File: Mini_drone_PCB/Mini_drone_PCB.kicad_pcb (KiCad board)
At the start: 2 copper layers, 45.7 x 42.9 mm, 56 parts, among them J1 XT30PW-M, Q1 SS8050, Q2 SS8050, Q3 AO3400, Q4 AO3400, Q5 AO3400, Q6 AO3400, Q7 AO4407A, SW1 SW_Push, SW2 Slide_switch, U1 TPS62085RLTR, U2 470nH 6.9mΩ, U3 ESP32-S3-MINI-1, U4 MPU-6050, U5 CH343P, U6 INA236AIDDFR, U7 USBLC6-2P6

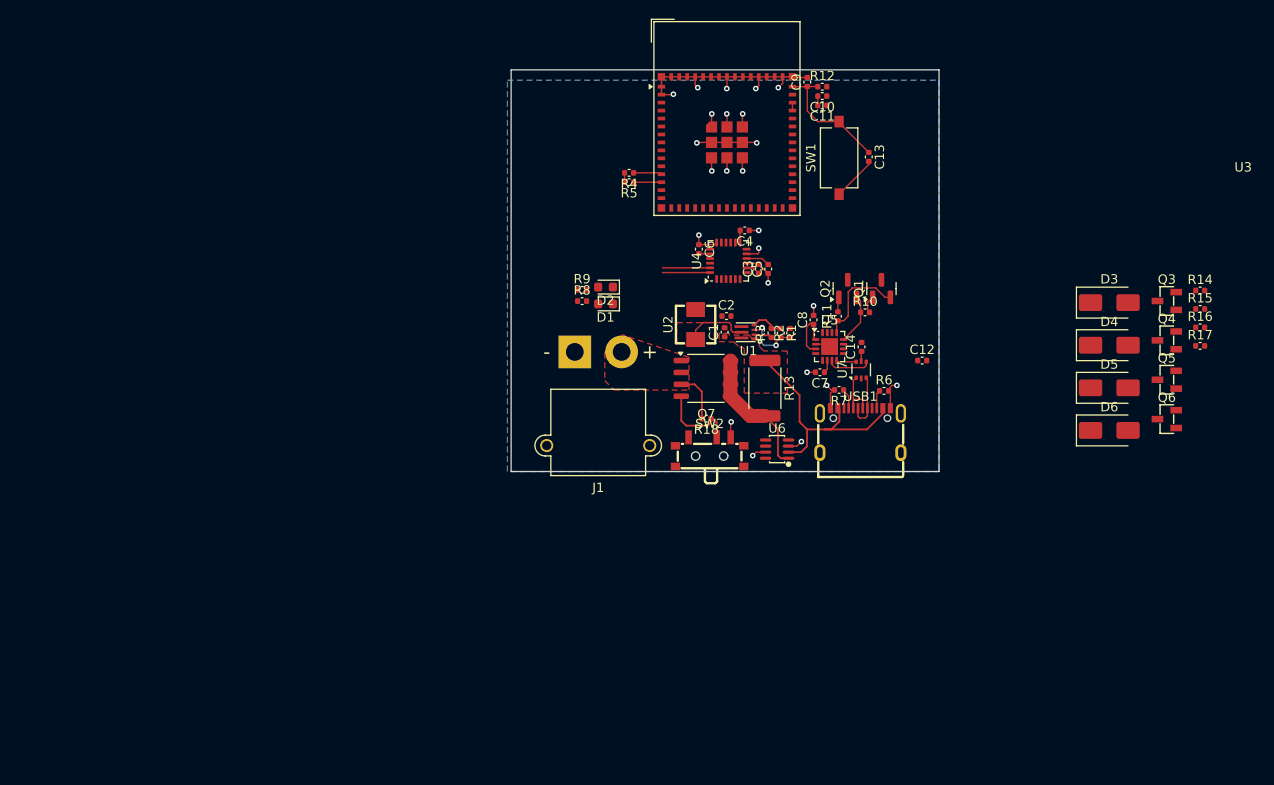
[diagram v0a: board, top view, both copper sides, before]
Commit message: update_sch_and_PCB
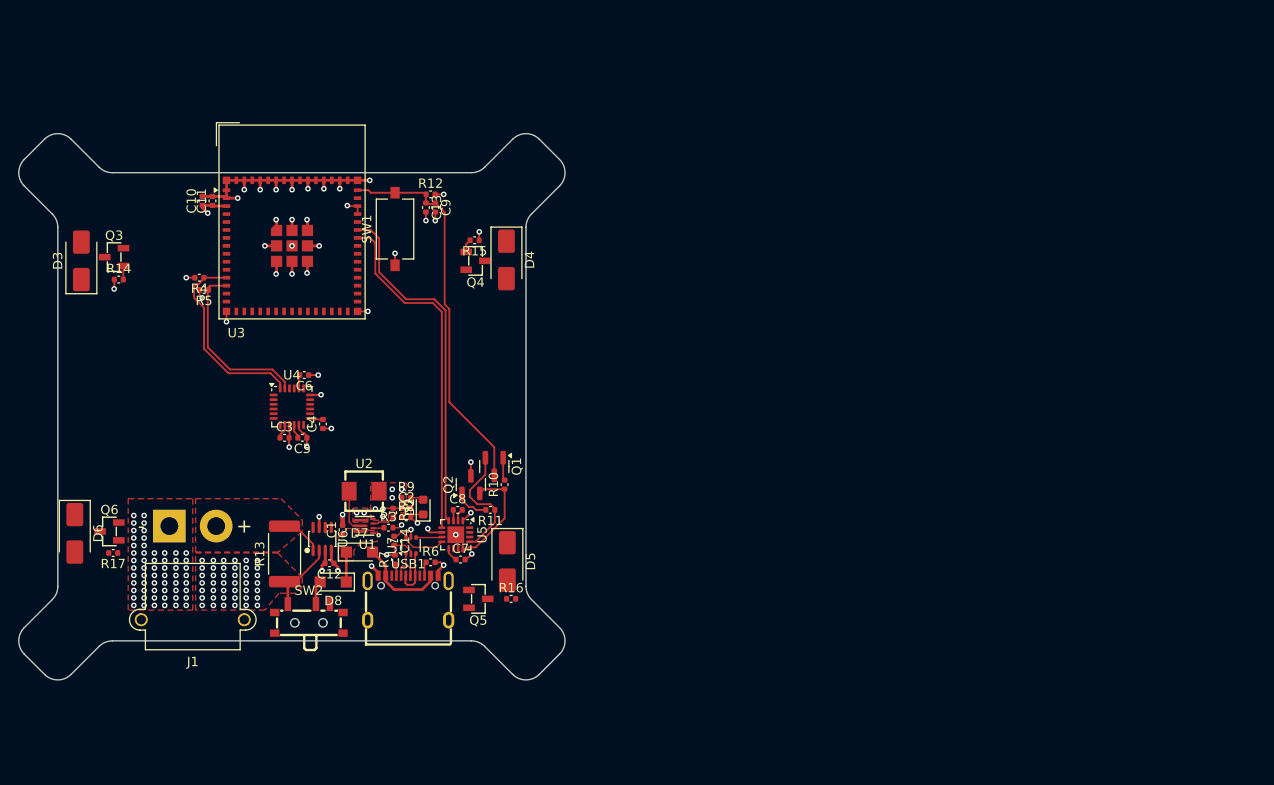
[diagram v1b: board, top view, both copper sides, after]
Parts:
- removed D1: VBAT LED, LED_SMD:LED_0603_1608Metric
- removed Q7: AO4407A, mini_drone:AO4407A
- removed R18: 10k, Capacitor_SMD:C_0402_1005Metric
- removed R8: 510, Capacitor_SMD:C_0402_1005Metric
- added D7: PMEG2010ER, Diode_SMD:Nexperia_CFP3_SOD-123W, F.Cu at (106.8, 115.1)
- added D8: PMEG2010ER, Diode_SMD:Nexperia_CFP3_SOD-123W, F.Cu at (104.0, 118.3)
- moved R17 118.2 mm to (80.5, 115.2), turned to 180 degrees
- moved R14 115.5 mm to (81.1, 86.0)
- moved Q6 113.6 mm to (80.1, 112.9)
- moved Q3 112.5 mm to (80.6, 83.6)
- moved D6 111.0 mm to (76.4, 113.1), turned to -90 degrees
- moved D3 109.9 mm to (77.1, 84.0), turned to 90 degrees
- moved R16 79.1 mm to (123.0, 120.1)
- moved R15 77.8 mm to (119.1, 81.8), turned to 180 degrees
- moved Q5 77.2 mm to (119.5, 120.1), turned to 180 degrees
- moved Q4 74.3 mm to (119.2, 84.0), turned to 180 degrees
- moved C10 67.1 mm to (90.0, 77.6), turned to 90 degrees
- moved D5 66.9 mm to (122.6, 116.1), turned to -90 degrees
- moved C12 66.9 mm to (103.6, 116.3), turned to 180 degrees
- moved C11 65.9 mm to (91.1, 77.6), turned to 90 degrees
- moved D4 65.0 mm to (122.5, 83.9), turned to -90 degrees
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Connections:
- C1 pad 1: +BATT -> +VIN
- C14 pad 1: +BATT -> +VBUS
- R13 pad 2: Net-(Q7-D) -> Net-(J1-+)
- SW2 pad 1: unconnected-(SW2-Pad1) -> +BATT
- SW2 pad 3: GND -> unconnected-(SW2-Pad3)
- U1 pad 1: +BATT -> +VIN
- U1 pad 7: +BATT -> +VIN
- U6 pad 1: Net-(Q7-D) -> Net-(J1-+)
- U7 pad 5: +BATT -> +VBUS
- USB1 pad 11: +BATT -> +VBUS
- USB1 pad 2: +BATT -> +VBUS
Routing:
- net /MCU/U0RXD: track 0.00 -> 37.7 mm
- net /MCU/U0TXD: track 0.00 -> 37.2 mm
- net /MCU/CHIP_PU: track 13.8 -> 41.1 mm
- net +BATT: track 27.1 -> 7.59 mm, vias 0 -> 42
- net Net-(Q7-D): track 14.4 -> 0.00 mm
- net /MCU/ESP_SDA: track 8.13 -> 21.2 mm
- net +VBUS: track 0.00 -> 12.7 mm, vias 0 -> 1
- net /MCU/ESP_SCL: track 8.07 -> 18.9 mm
- net +3V3: track 14.6 -> 21.9 mm, vias 0 -> 14
- net Net-(D8-A): track 8.93 -> 2.55 mm
- net /MCU/DTR: track 5.51 -> 11.8 mm
- net GND: track 69.6 -> 74.1 mm, vias 24 -> 100
- net Net-(U1-FB): track 6.28 -> 2.43 mm, vias 2 -> 0
- net +VIN: track 0.00 -> 2.90 mm
- net /MCU/RTS: track 10.3 -> 13.1 mm
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- added copper zone on F.Cu, net +3V3
- added copper zone on F.Cu, net +VIN
- added copper zone on F.Cu, net GND
- removed copper zone on B.Cu, net GND
- removed copper zone on F.Cu, net Net-(U1-SW)
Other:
- board size 45.7 x 42.9 mm -> 58.3 x 58.3 mm

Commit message: Route_Finished
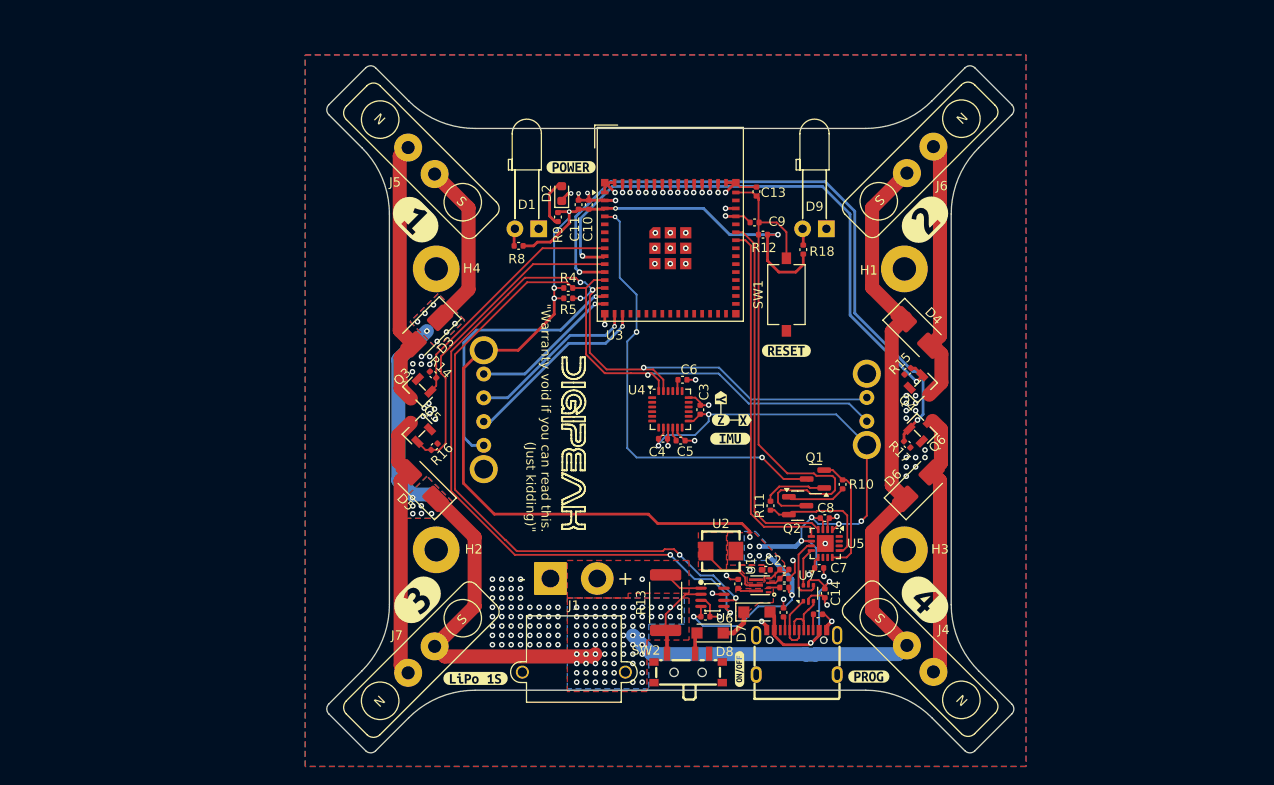
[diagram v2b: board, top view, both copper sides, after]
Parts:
- added D1: LED, LED_THT:LED_D3.0mm_Horizontal_O6.35mm_Z2.0mm, F.Cu at (125.9, 80.6)
- added D9: LED, LED_THT:LED_D3.0mm_Horizontal_O6.35mm_Z2.0mm, F.Cu at (156.7, 80.6)
- added H1: MountingHole_Pad, MountingHole:MountingHole_2.5mm_Pad, F.Cu at (165.0, 84.9)
- added H2: MountingHole_Pad, MountingHole:MountingHole_2.5mm_Pad, F.Cu at (115.0, 114.9)
- added H3: MountingHole_Pad, MountingHole:MountingHole_2.5mm_Pad, F.Cu at (165.0, 114.9)
- added H4: MountingHole_Pad, MountingHole:MountingHole_2.5mm_Pad, F.Cu at (115.0, 84.9)
- added J2: VL53L1X ToF Pogo, mini_drone:POGO 4Pin Pitch 2.54, B.Cu at (155.9, 101.1)
- added J3: PMW3901 Optical Flow Pogo, mini_drone:POGO 6Pin Pitch 2.54, B.Cu at (125.2, 96.1)
- added J4: Motor4_Pogo, mini_drone:POGO 2Pin Pitch 4, F.Cu at (169.9, 122.6)
- added J5: Motor1_Pogo, mini_drone:POGO 2Pin Pitch 4, F.Cu at (110.2, 77.2)
- added J6: Motor2_Pogo, mini_drone:POGO 2Pin Pitch 4, F.Cu at (162.8, 70.0)
- added J7: Motor3_Pogo, mini_drone:POGO 2Pin Pitch 4, F.Cu at (117.3, 129.8)
- added R18: 510, Capacitor_SMD:C_0402_1005Metric, F.Cu at (154.2, 82.8)
- added R8: 510, Capacitor_SMD:C_0402_1005Metric, F.Cu at (123.8, 82.4)
- added kibuzzard-696EF072: G***, kibuzzard-696EF072, F.Cu at (119.2, 128.6)
- added kibuzzard-696EF0B2: G***, kibuzzard-696EF0B2, F.Cu at (161.2, 128.4)
- added kibuzzard-696EF12B: G***, kibuzzard-696EF12B, F.Cu at (112.8, 79.6)
- added kibuzzard-696EF142: G***, kibuzzard-696EF142, F.Cu at (167.2, 79.6)
- added kibuzzard-696EF14F: G***, kibuzzard-696EF14F, F.Cu at (113.0, 120.2)
- added kibuzzard-696EF15F: G***, kibuzzard-696EF15F, F.Cu at (167.2, 120.2)
- added kibuzzard-696EF1CC: G***, kibuzzard-696EF1CC, F.Cu at (147.4, 127.6)
- added kibuzzard-696EF1EE: G***, kibuzzard-696EF1EE, F.Cu at (152.4, 93.6)
- added kibuzzard-696EF202: G***, kibuzzard-696EF202, F.Cu at (129.4, 74.0)
- added kibuzzard-696EF46D: G***, kibuzzard-696EF46D, B.Cu at (124.4, 100.0)
- added kibuzzard-696EF488: G***, kibuzzard-696EF488, B.Cu at (156.8, 100.0)
- added kibuzzard-696EFAC1: G***, kibuzzard-696EFAC1, F.Cu at (148.0, 101.0)
- added kibuzzard-696EFAE6: G***, kibuzzard-696EFAE6, F.Cu at (145.4, 98.6)
- added kibuzzard-696EFB18: G***, kibuzzard-696EFB18, F.Cu at (145.4, 101.0)
- added kibuzzard-696EFB3D: G***, kibuzzard-696EFB3D, F.Cu at (146.4, 103.0)
- R9: value 220 -> 510
- moved D6 90.2 mm to (166.5, 108.0), turned to 45 degrees
- moved Q6 87.5 mm to (166.9, 101.9), turned to -135 degrees
- moved R17 85.6 mm to (165.3, 103.6), turned to 135 degrees
- moved Q4 49.6 mm to (166.9, 97.6), turned to 135 degrees
- moved R15 48.3 mm to (165.3, 95.8), turned to 45 degrees
- moved C14 46.3 mm to (156.5, 119.5)
- moved D4 44.5 mm to (166.3, 91.7), turned to -45 degrees
- moved C3 44.5 mm to (143.2, 99.9), turned to 90 degrees
- moved D7 42.9 mm to (149.2, 121.5)
- moved R3 42.8 mm to (152.2, 118.9)
- moved U7 42.8 mm to (154.8, 119.5)
- moved U1 42.7 mm to (149.8, 118.7)
- moved C1 42.6 mm to (147.2, 118.5)
- moved SW1 42.4 mm to (152.4, 87.6)
- moved R1 42.2 mm to (152.2, 117.0), turned to 0 degrees
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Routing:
- net +3V3: track 21.9 -> 199.0 mm, vias 14 -> 20
- net +BATT: track 7.59 -> 173.6 mm, vias 42 -> 89
- net /MCU/ESP_SCL: track 18.9 -> 117.5 mm, vias 0 -> 6
- net /MCU/ESP_SDA: track 21.2 -> 113.3 mm, vias 0 -> 3
- net /MCU/Motor4_PWM: track 0.00 -> 70.0 mm, vias 0 -> 2
- net /MCU/Motor2_PWM: track 1.42 -> 61.3 mm, vias 0 -> 2
- net /MCU/GPIO0: track 1.46 -> 48.0 mm, vias 1 -> 3
- net /MCU/Motor3_PWM: track 0.00 -> 34.8 mm
- net /MCU/ESP_CS: track 0.00 -> 29.7 mm, vias 0 -> 1
- net Net-(D3-A): track 0.00 -> 28.8 mm
- net Net-(D5-A): track 0.00 -> 28.4 mm
- net Net-(D6-A): track 0.00 -> 28.2 mm
- net Net-(D4-A): track 0.00 -> 28.1 mm
- net /MCU/Motor1_PWM: track 1.46 -> 26.9 mm
- net /MCU/ESP_MISO: track 0.00 -> 20.4 mm, vias 0 -> 1
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- added copper zone on B.Cu, net +3V3
- added copper zone on B.Cu, net +BATT
- added copper zone on B.Cu, net GND
- added copper zone on F.Cu, net Net-(U1-SW)
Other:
- board size 58.3 x 58.3 mm -> 73.4 x 73.4 mm
- board text added: "Offset"
- board text added: "{dblquote}Warranty void if you can read this. (Just kidding){dblquote}"

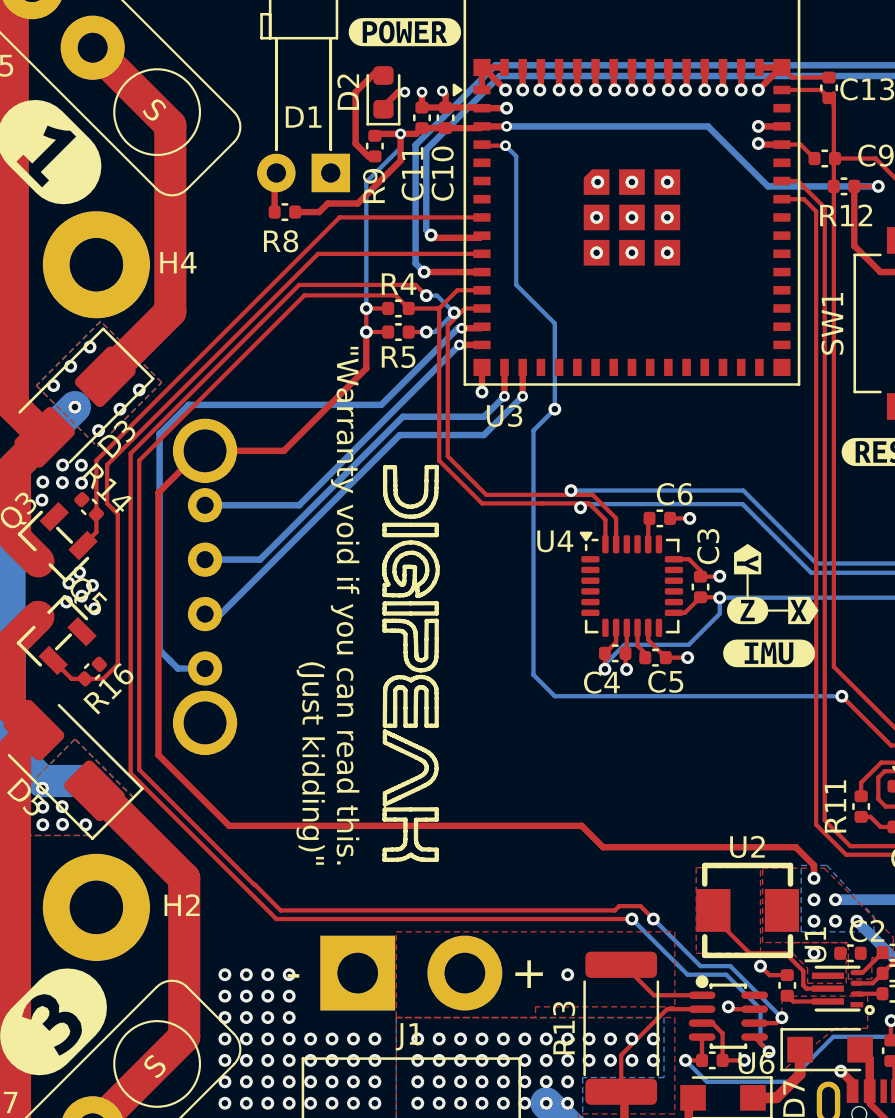
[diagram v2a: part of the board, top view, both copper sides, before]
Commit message: Verified and Finished
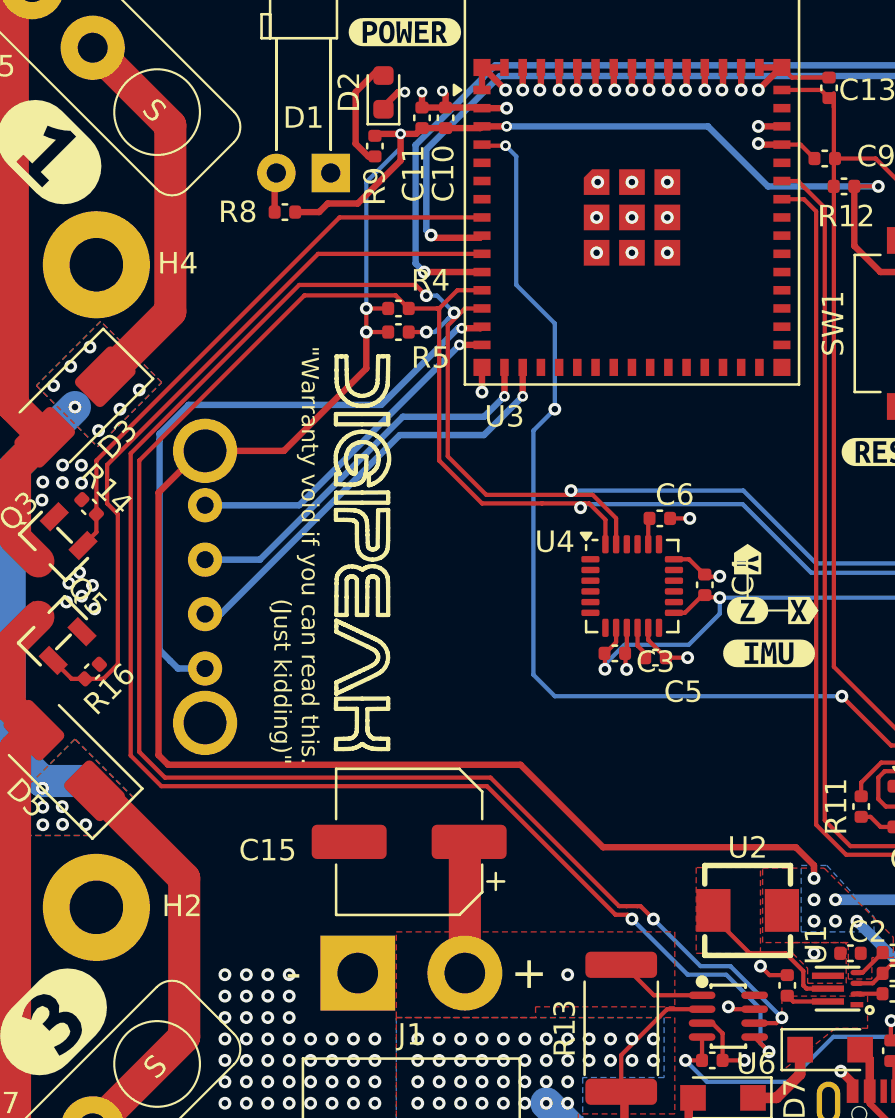
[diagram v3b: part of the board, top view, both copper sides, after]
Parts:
- added C15: 220uF, Capacitor_SMD:CP_Elec_6.3x5.4, F.Cu at (129.6, 111.8)
- moved C4 5.26 mm to (143.4, 99.8), turned to -90 degrees
- moved C3 5.06 mm to (139.2, 103.0), turned to 0 degrees
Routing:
- net Net-(J1-+): track 4.36 -> 10.6 mm
- net /MCU/ESP_SDA: track 113.3 -> 112.6 mm
